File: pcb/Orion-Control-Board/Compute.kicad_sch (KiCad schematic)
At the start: 20 parts, among them J10 POWER, J2 NUCLEO64_CN7, J3 JETSON_ORIN_NANO_DEVKIT_GPIO, J4 5V Select Socket, J5 5V Select Jumper, J6 NUCLEO64_CN10, J7 I2C 1, J8 I2C 3, J9 UART

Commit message: Route more
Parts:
- J9: footprint digikey-footprints:PinHeader_1x3_P2.54_Drill1.1mm -> Connector_PinHeader_2.54mm:PinHeader_1x03_P2.54mm_Vertical
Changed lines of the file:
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@@
 			)
 		)
-		(property "Footprint" "digikey-footprints:PinHeader_1x3_P2.54_Drill1.1mm"
+		(property "Footprint" "Connector_PinHeader_2.54mm:PinHeader_1x03_P2.54mm_Vertical"
 			(at 175.26 72.39 0)
 			(effects

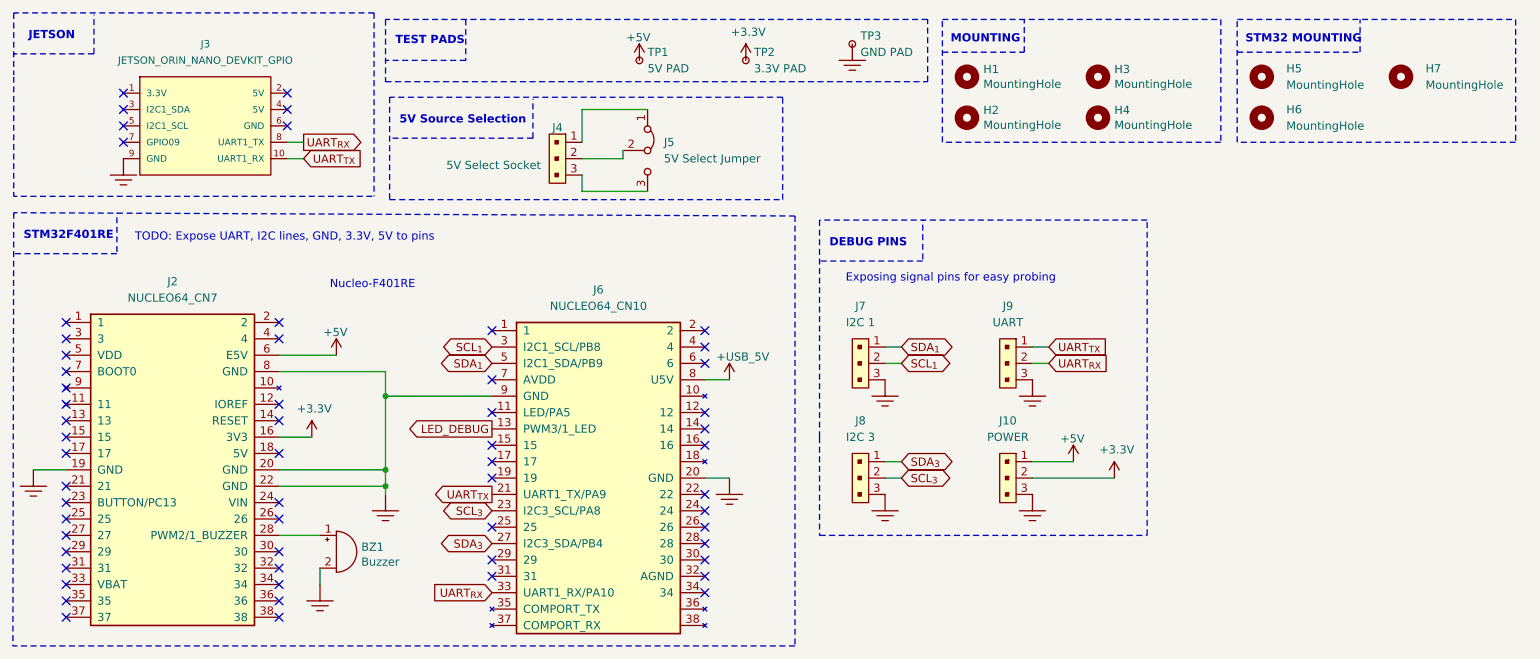
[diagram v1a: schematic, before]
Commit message: Route most traces
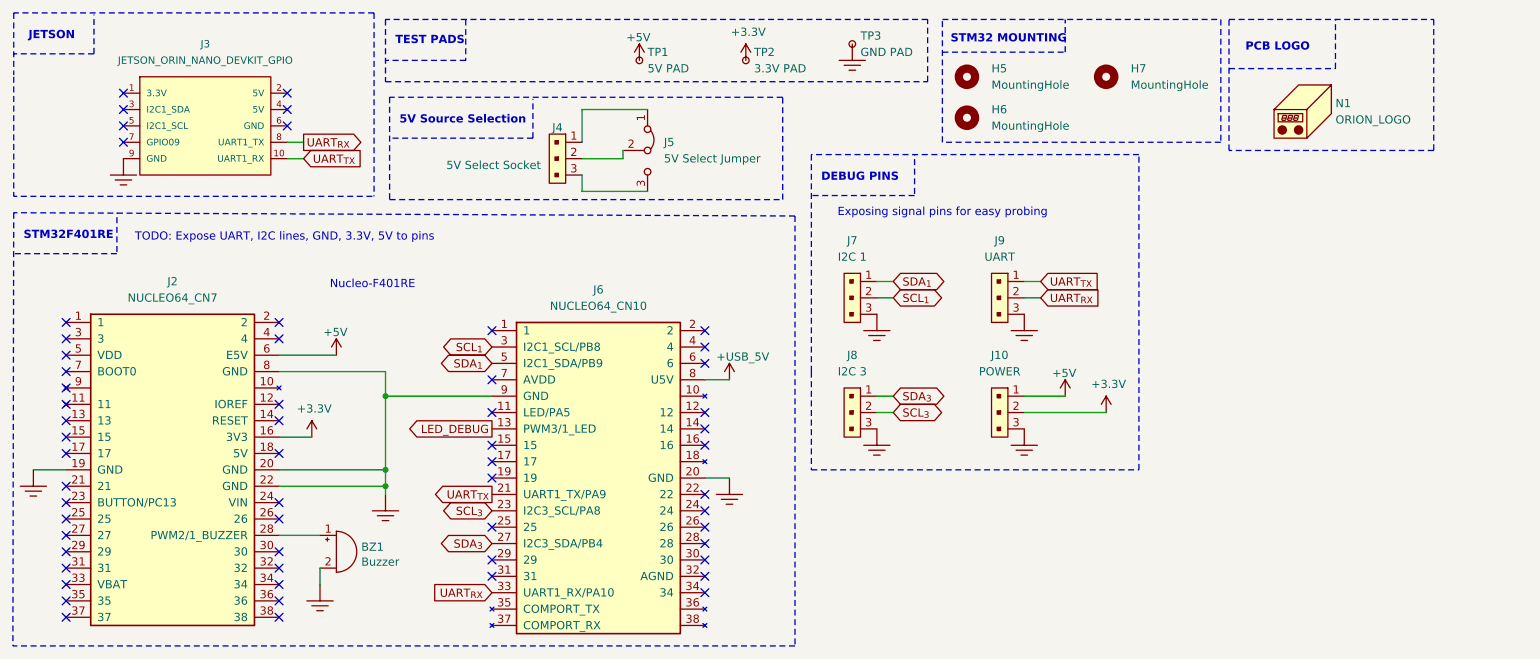
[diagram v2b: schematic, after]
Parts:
- removed H1, H2, H3, H4: MountingHole, MountingHole:MountingHole_3.2mm_M3_Pad, symbol Mechanical:MountingHole
- added N1: ORION_LOGO, Orion-Logo:Orion-Logo-20mm, symbol Mechanical:Housing
- J10, J7, J8: footprint digikey-footprints:PinHeader_1x3_P2.54_Drill1.1mm -> Connector_PinHeader_2.54mm:PinHeader_1x03_P2.54mm_Vertical
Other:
- note added: "PCB LOGO"
- note removed: "MOUNTING"
- moved on the sheet: H5, H6, H7, J10, J7, J8, J9
